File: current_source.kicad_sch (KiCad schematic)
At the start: 3 parts, among them Q1 NMOS

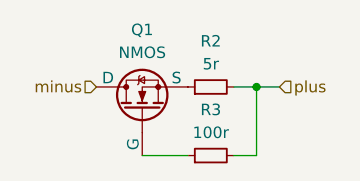
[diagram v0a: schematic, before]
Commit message: pretty neat neg needs testing
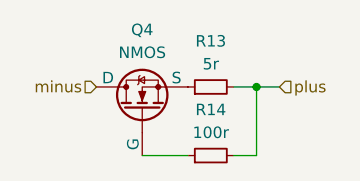
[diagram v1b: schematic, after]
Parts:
- renumbered Q1 to Q4, R2 to R13, R3 to R14
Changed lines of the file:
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@@
 		(dnp no)
 		(fields_autoplaced yes)
-		(property "Reference" "Q1"
+		(property "Reference" "Q4"
 			(at 133.35 91.44 90)
 			(effects
@@
 		(dnp no)
 		(fields_autoplaced yes)
-		(property "Reference" "R3"
+		(property "Reference" "R14"
 			(at 140.97 100.33 90)
 			(effects
@@
 		(dnp no)
 		(fields_autoplaced yes)
-		(property "Reference" "R2"
+		(property "Reference" "R13"
 			(at 140.97 92.71 90)
 			(effects
